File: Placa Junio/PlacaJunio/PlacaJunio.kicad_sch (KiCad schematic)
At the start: 13 parts, among them IC1 LC86LICMD, J5 Terminal P3, J6 Terminal P4, Q4 IRLML0030, U5 TSR2-2433N

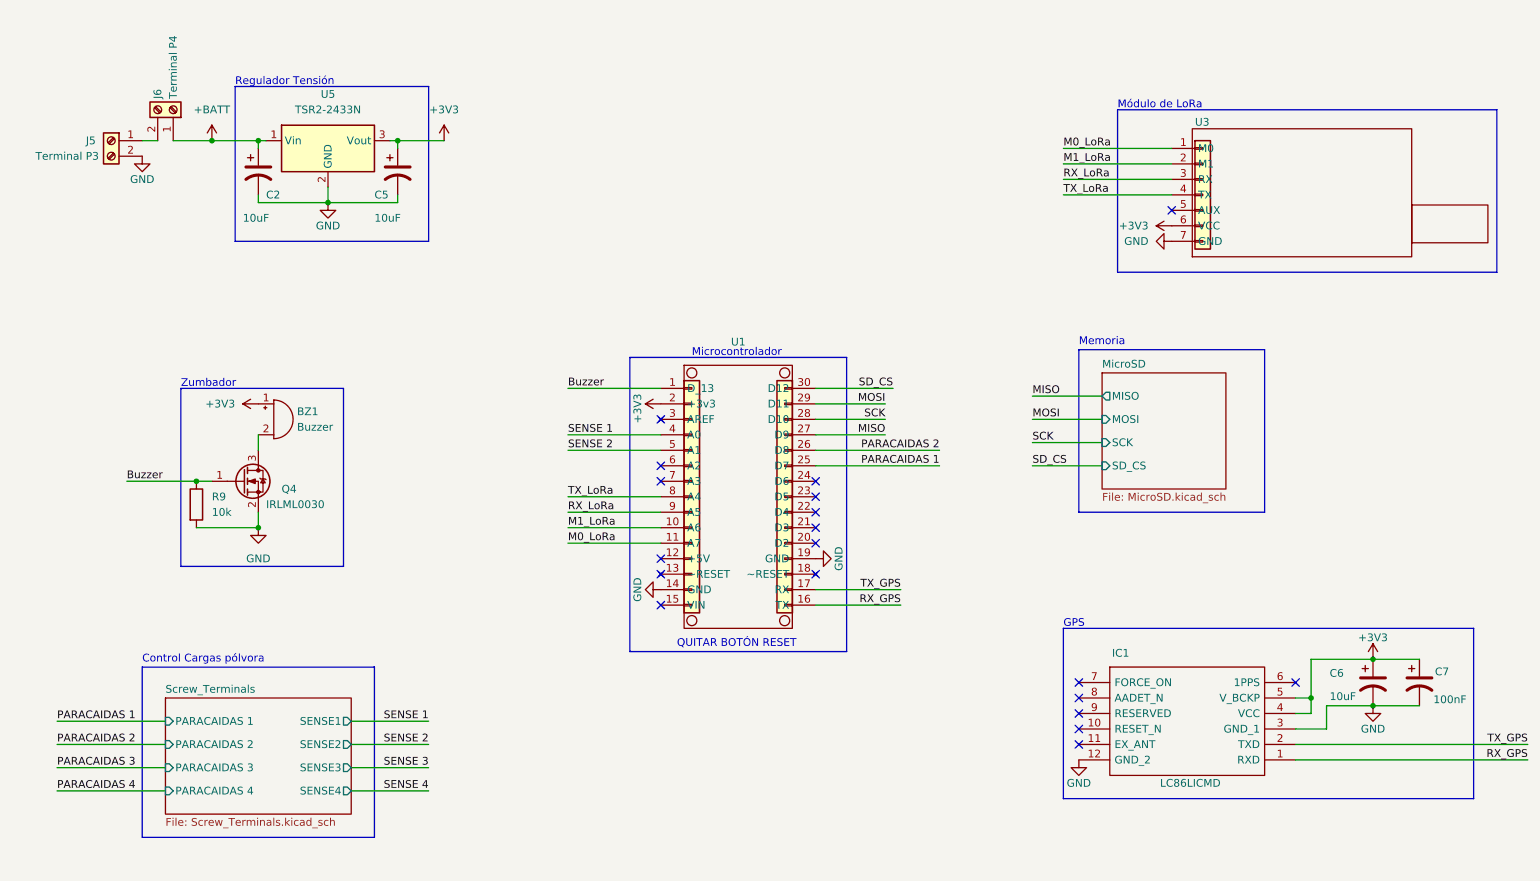
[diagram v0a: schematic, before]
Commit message: Primera versión definitiva
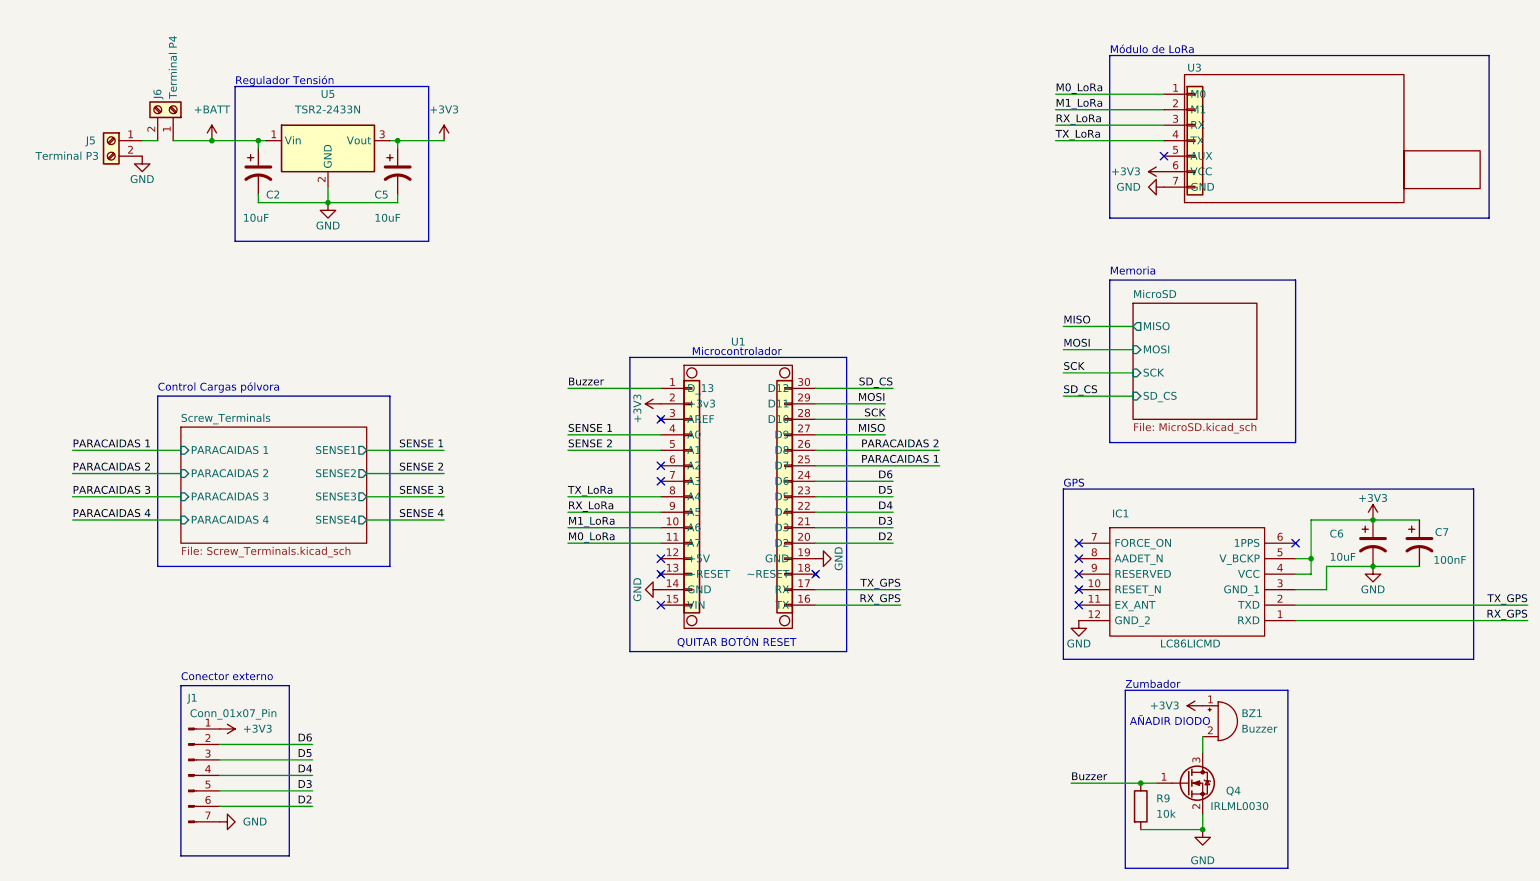
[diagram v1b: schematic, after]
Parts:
- added J1: Conn_01x07_Pin, Connector_PinHeader_2.54mm:PinHeader_1x07_P2.54mm_Vertical, symbol Connector:Conn_01x07_Pin
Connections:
- net +3V3: now also J1.1 (Pin_1)
- net GND: now also J1.7 (Pin_7)
- net D2: now reaches U1.20 (D2)
- net D2: now also J1.6 (Pin_6)
- net D3: now reaches U1.21 (D3)
- net D3: now also J1.5 (Pin_5)
- net D4: now reaches U1.22 (D4)
- net D4: now also J1.4 (Pin_4)
- net D5: now reaches U1.23 (D5)
- net D5: now also J1.3 (Pin_3)
- net D6: now reaches U1.24 (D6)
- net D6: now also J1.2 (Pin_2)
- no-connect marks 19 -> 14
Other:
- note added: "AÑADIR DIODO"
- note added: "Conector externo"
- moved on the sheet: BZ1, C6, C7, IC1, Q4, R9, U3
